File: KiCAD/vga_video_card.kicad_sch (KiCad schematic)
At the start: 5 parts, among them J1 DE15_Socket_HighDensity, SW1 rst_btn, U27 74HC04, Y1 10MHz

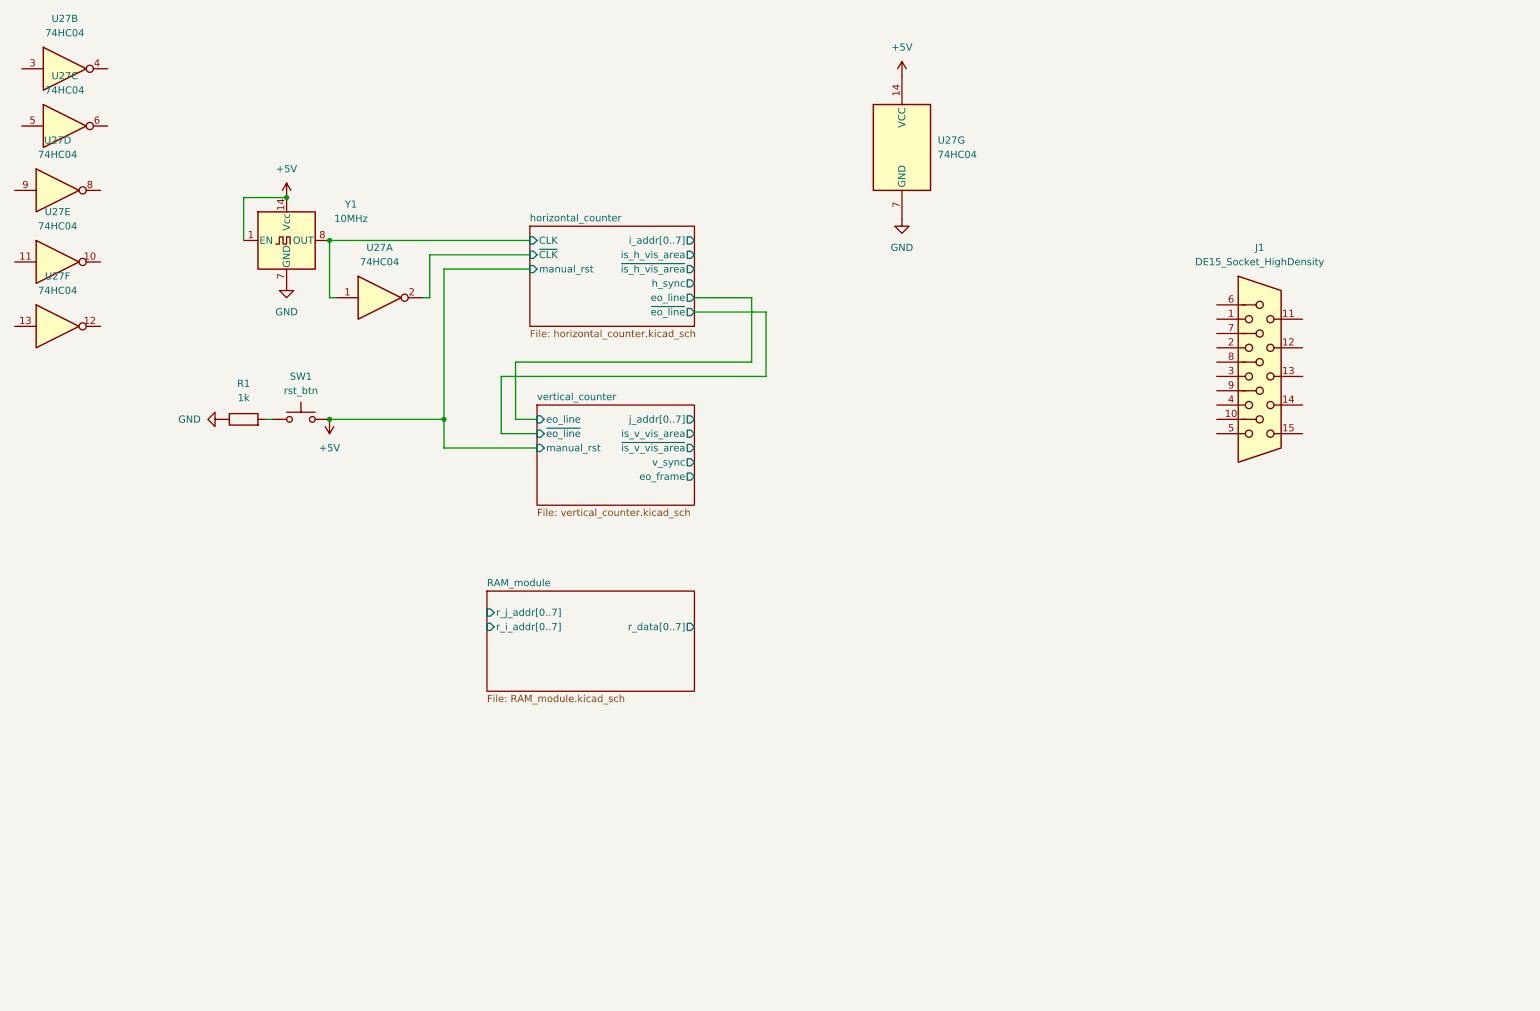
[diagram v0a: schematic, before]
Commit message: finished schematics and footprint assignments; need to figure out +5v connection issue
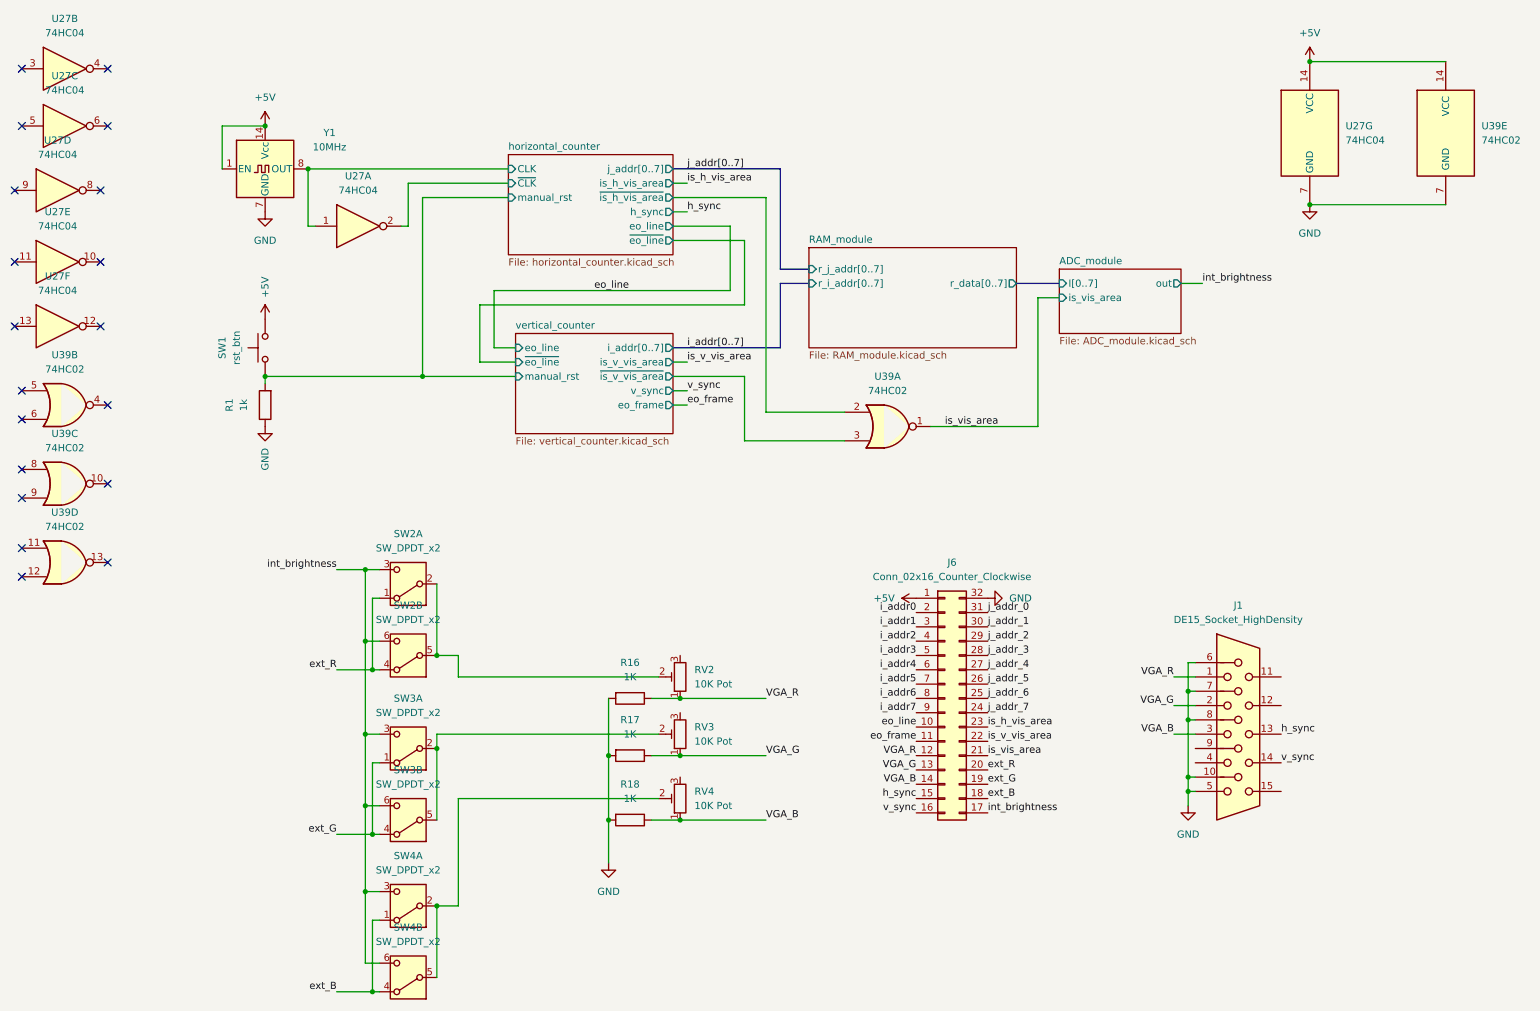
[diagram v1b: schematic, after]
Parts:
- added J6: Conn_02x16_Counter_Clockwise, Connector_PinSocket_2.54mm:PinSocket_2x16_P2.54mm_Vertical, symbol Connector_Generic:Conn_02x16_Counter_Clockwise
- added R16, R17, R18: 1K, Resistor_THT:R_Axial_DIN0207_L6.3mm_D2.5mm_P7.62mm_Horizontal, symbol Device:R
- added RV2, RV3, RV4: 10K Pot, Potentiometer_THT:Potentiometer_Vishay_T73YP_Vertical, symbol Device:R_Potentiometer_Trim
- added SW2, SW3, SW4: SW_DPDT_x2, Button_Switch_THT:SW_CK_JS202011CQN_DPDT_Straight, symbol Switch:SW_DPDT_x2
- added U39: 74HC02, Package_DIP:DIP-14_W7.62mm, symbol 74xx:74HC02
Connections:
- net +5V: now also J6.1 (Pin_1), U39.14 (VCC)
- net GND: now also J1.10, J1.5, J1.6, J1.7, J1.8, J6.32 (Pin_32), R16.2, R17.2, R18.2, U39.7 (GND)
- net horizontal_counter/~{is_h_vis_area}: now also U39.2
- net vertical_counter/~{is_v_vis_area}: now also U39.3
- net VGA_R: now reaches J1.1
- net VGA_R: now also J6.12 (Pin_12), R16.1, RV2.1
- net h_sync: now reaches J1.13
- net h_sync: now also J6.15 (Pin_15)
- net v_sync: now reaches J1.14
- net v_sync: now also J6.16 (Pin_16)
- net VGA_G: now reaches J1.2
- net VGA_G: now also J6.13 (Pin_13), R17.1, RV3.1
- net VGA_B: now reaches J1.3
- net VGA_B: now also J6.14 (Pin_14), R18.1, RV4.1
- net horizontal_counter/manual_rst: now reaches R1.2, SW1.1
- new net: RV2.2, SW2.2 (B), SW2.5 (B)
- new net: RV4.2, SW4.2 (B), SW4.5 (B)
- new net: RV3.2, SW3.2 (B), SW3.5 (B)
- new net eo_frame: J6.11 (Pin_11)
- new net eo_line: J6.10 (Pin_10)
- new net ext_B: J6.18 (Pin_18), SW4.1 (A), SW4.4 (A)
- new net ext_G: J6.19 (Pin_19), SW3.1 (A), SW3.4 (A)
- new net ext_R: J6.20 (Pin_20), SW2.1 (A), SW2.4 (A)
- new net i_addr0: J6.2 (Pin_2)
- new net i_addr1: J6.3 (Pin_3)
- new net i_addr2: J6.4 (Pin_4)
- new net i_addr3: J6.5 (Pin_5)
- new net i_addr4: J6.6 (Pin_6)
- new net i_addr5: J6.7 (Pin_7)
- new net i_addr6: J6.8 (Pin_8)
- new net i_addr7: J6.9 (Pin_9)
- new net int_brightness: J6.17 (Pin_17), SW2.3 (C), SW2.6 (C), SW3.3 (C), SW3.6 (C), SW4.3 (C), SW4.6 (C)
- new net is_h_vis_area: J6.23 (Pin_23)
- new net is_v_vis_area: J6.22 (Pin_22)
- new net is_vis_area: J6.21 (Pin_21), U39.1
- new net j_addr_0: J6.31 (Pin_31)
- new net j_addr_1: J6.30 (Pin_30)
- new net j_addr_2: J6.29 (Pin_29)
- new net j_addr_3: J6.28 (Pin_28)
- new net j_addr_4: J6.27 (Pin_27)
- new net j_addr_5: J6.26 (Pin_26)
- new net j_addr_6: J6.25 (Pin_25)
- new net j_addr_7: J6.24 (Pin_24)
- no-connect marks 0 -> 19
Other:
- added sheet ADC_module (ADC_module.kicad_sch)
- sheet horizontal_counter ports: added j_addr[0..7]; removed i_addr[0..7]
- sheet vertical_counter ports: added i_addr[0..7]; removed j_addr[0..7]
- moved on the sheet: J1, R1, SW1, U27A, U27G, Y1
